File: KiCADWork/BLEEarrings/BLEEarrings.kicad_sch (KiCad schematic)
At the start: 16 parts, among them Q1 DMP3013SFV, SW1 PB22E06071, U1 XB6096I2SV, U2 MCP73831T-2ACI/OT, U3 GT-USB-7010ASV, U4 2.0MM-2P WZ MS

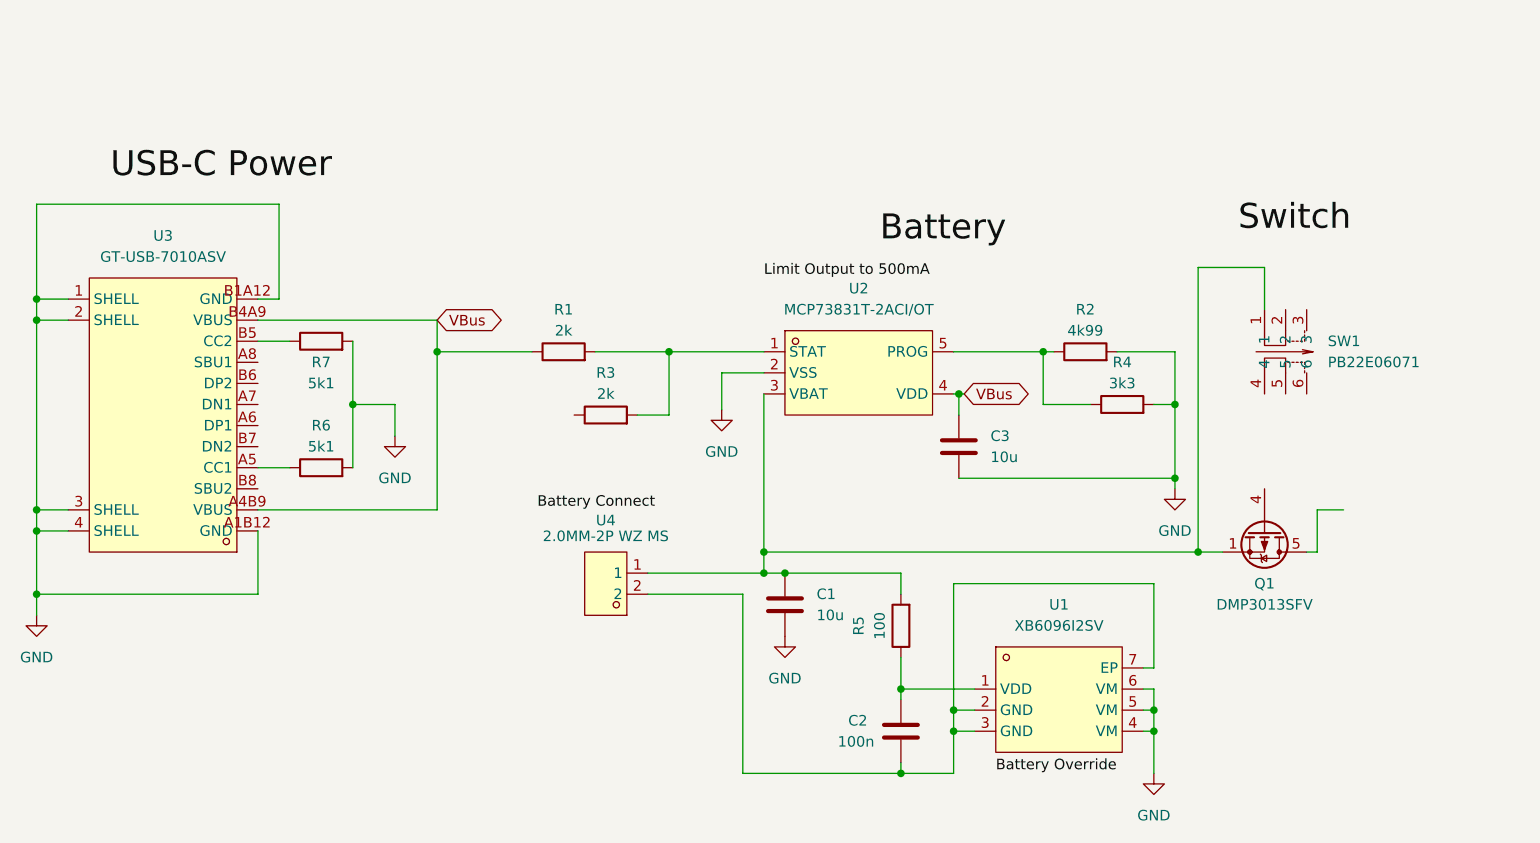
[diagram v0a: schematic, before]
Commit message: More KiCAD Work
More KiCAD work complete
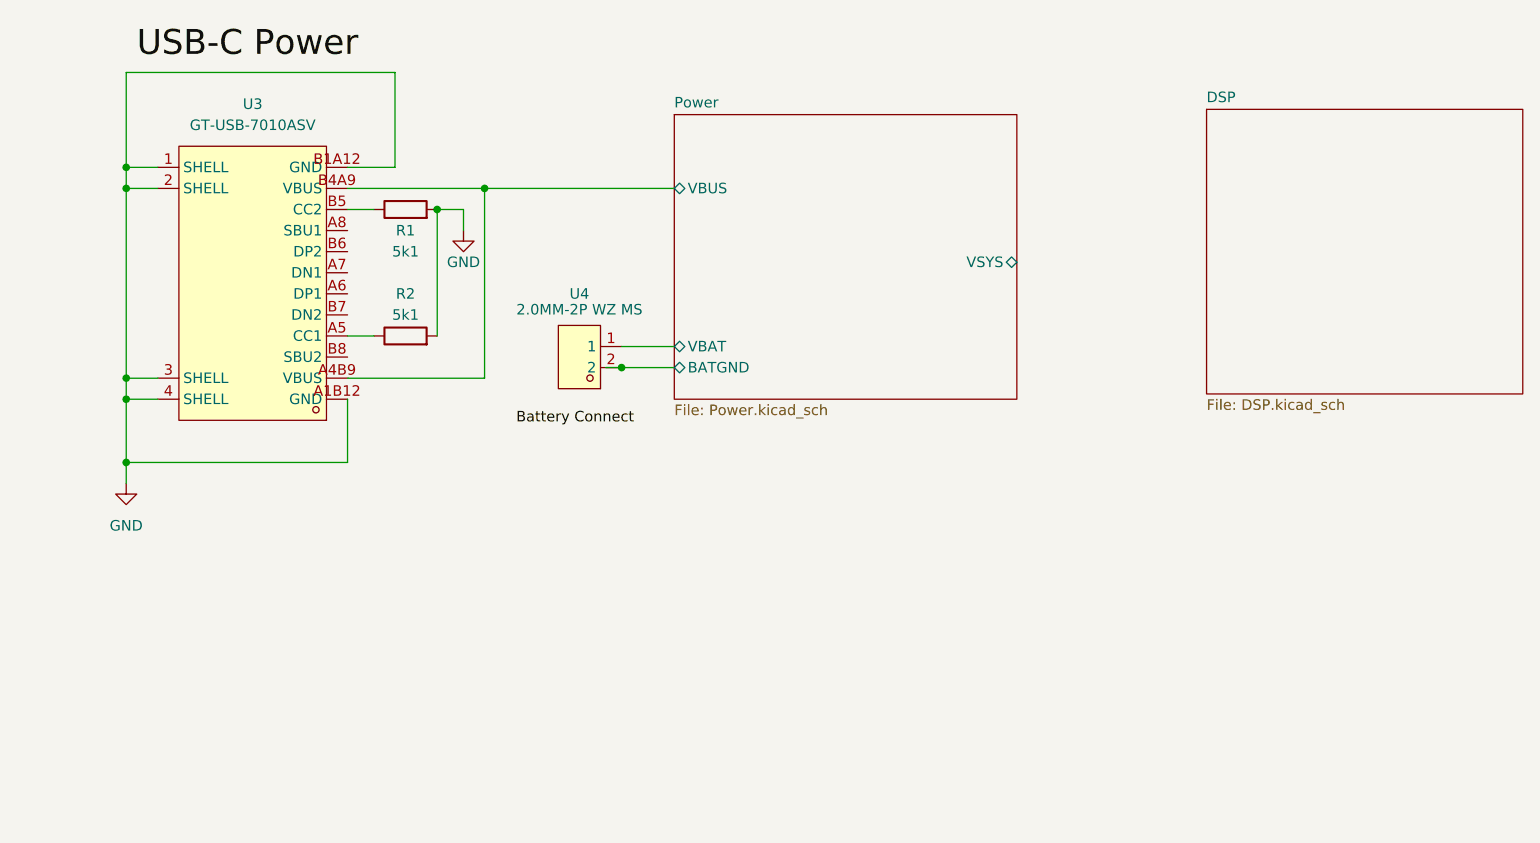
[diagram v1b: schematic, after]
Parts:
- removed C1, C3: 10u, Capacitor_SMD:C_0402_1005Metric_Pad0.74x0.62mm_HandSolder, symbol Device:C
- removed C2: 100n, Capacitor_SMD:C_0402_1005Metric_Pad0.74x0.62mm_HandSolder, symbol Device:C
- removed Q1: DMP3013SFV, Package_SON:Diodes_PowerDI3333-8, symbol Transistor_FET:DMP3013SFV
- removed R3: 2k, Resistor_SMD:R_0402_1005Metric, symbol Device:R
- removed R4: 3k3, Resistor_SMD:R_0402_1005Metric, symbol Device:R
- removed R5: 100, Resistor_SMD:R_0402_1005Metric, symbol Device:R
- removed R6, R7: 5k1, Resistor_SMD:R_0402_1005Metric, symbol Device:R
- removed SW1: PB22E06071, easyeda2kicad:SW-TH_6P-L5.8-W5.8-P2.00-LS4.5_PB22E06371-0625, symbol easyeda2kicad:PB22E06071
- removed U1: XB6096I2SV, easyeda2kicad:WDFN-6_L2.0-W2.0-P0.65-BL-EP, symbol easyeda2kicad:XB6096I2SV
- removed U2: MCP73831T-2ACI/OT, easyeda2kicad:SOT-23-5_L3.0-W1.7-P0.95-LS2.8-BL, symbol easyeda2kicad:MCP73831T-2ACI_OT
- R1: value 2k -> 5k1
- R2: value 4k99 -> 5k1
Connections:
- net GND: now also R1.2
- net Power/VBAT: now reaches U4.1
- net Power/BATGND: now reaches U4.2
- net at U3.A5 (CC1): now also R2.1
- net at U3.B5 (CC2): now also R1.1
- net VBus renamed Power/VBUS
- net Power/VBUS: no longer R1.1
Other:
- added sheet DSP (DSP.kicad_sch)
- added sheet Power (Power.kicad_sch)
- moved on the sheet: U3, U4
